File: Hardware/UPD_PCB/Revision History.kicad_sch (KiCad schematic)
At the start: 0 parts

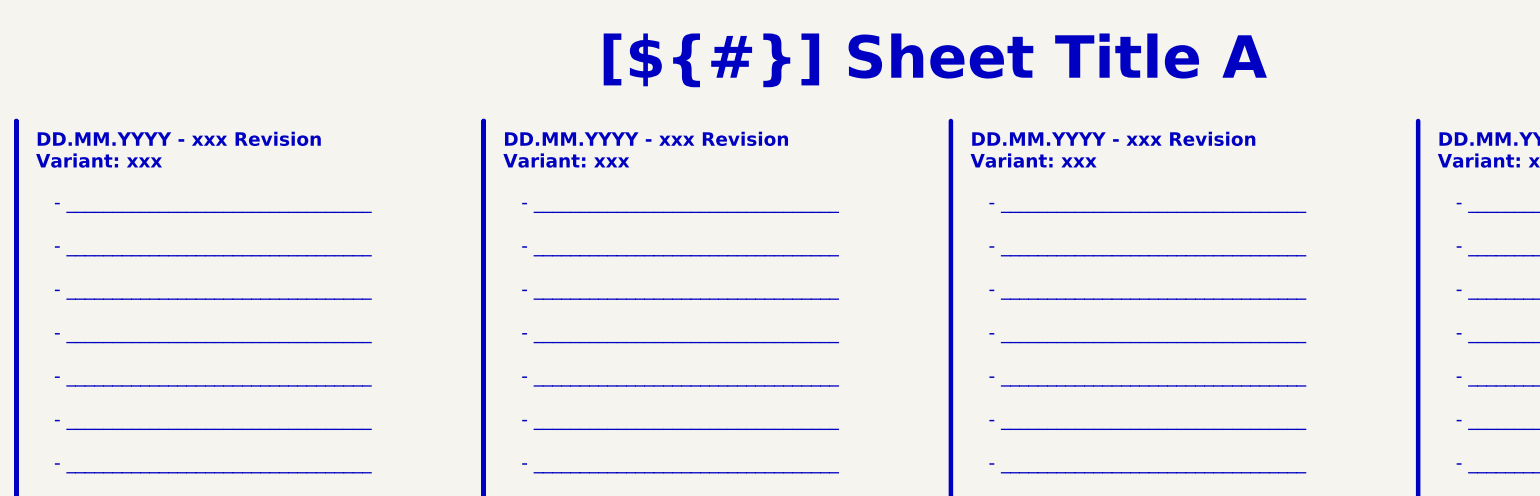
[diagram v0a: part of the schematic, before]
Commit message: Finalized version V1.0
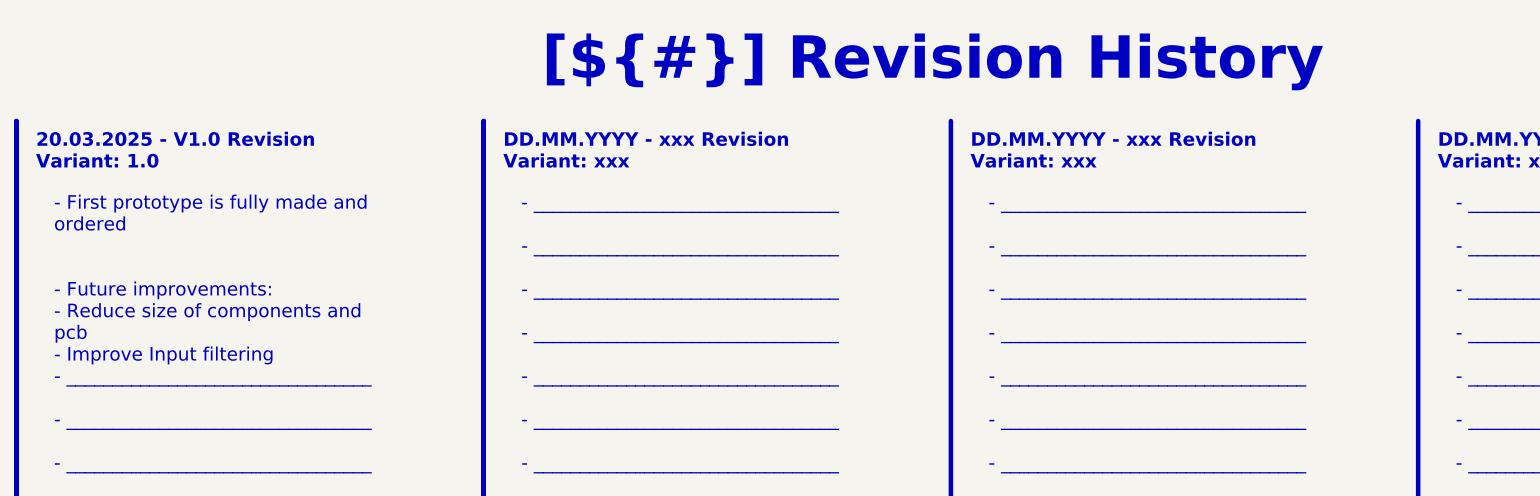
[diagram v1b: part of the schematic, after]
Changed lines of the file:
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@@
 		)
 	)
-	(text_box "[${#}] ${TITLE}"
+	(text_box "[${#}] Revision History\n"
 		(exclude_from_sim no)
 		(at 80.01 16.51 0)
@@
 		)
 	)
-	(text_box "- _________________________________\n\n- _________________________________\n\n- _________________________________\n\n- _________________________________\n\n- _________________________________\n\n- _________________________________\n\n- _________________________________\n\n- _________________________________\n\n- _________________________________\n\n- _________________________________\n\n- _________________________________\n\n- _________________________________\n\n- _________________________________\n\n- _________________________________\n\n- _________________________________\n\n- _________________________________\n\n- _________________________________"
+	(text_box "- First prototype is fully made and ordered\n\n\n- Future improvements:\n- Reduce size of components and pcb\n- Improve Input filtering\n- _________________________________\n\n- _________________________________\n\n- _________________________________\n\n- _________________________________\n\n- _________________________________\n\n- _________________________________\n\n- _________________________________\n\n- _________________________________\n\n- _________________________________\n\n- _________________________________\n\n- _________________________________\n\n- _________________________________\n\n- _________________________________"
 		(exclude_from_sim no)
 		(at 22.86 40.64 0)
@@
 		)
 	)
-	(text_box "DD.MM.YYYY - xxx Revision\nVariant: xxx"
+	(text_box "20.03.2025 - V1.0 Revision\nVariant: 1.0"
 		(exclude_from_sim no)
 		(at 20.32 31.75 0)

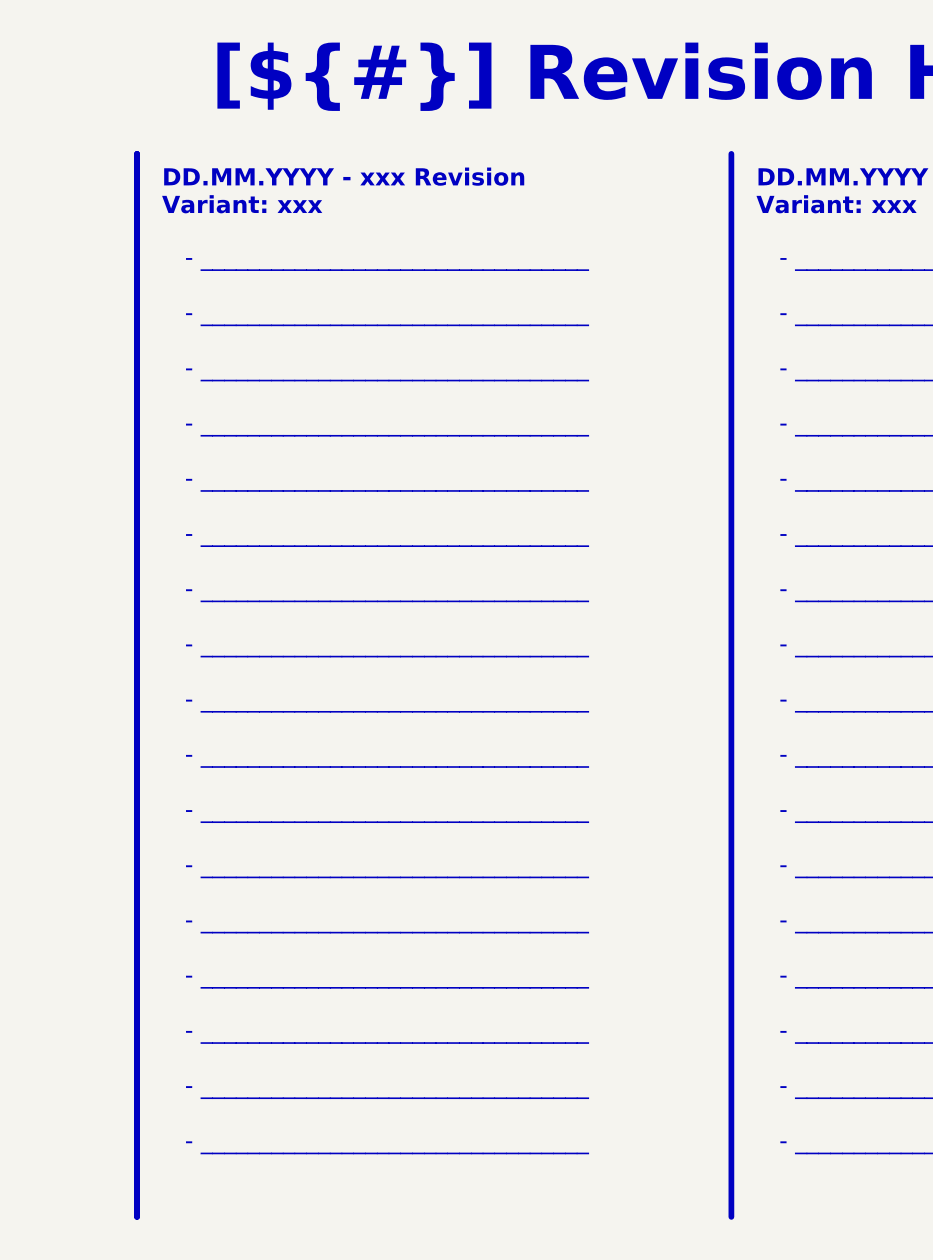
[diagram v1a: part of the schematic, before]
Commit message: Version 1.1 of PCB
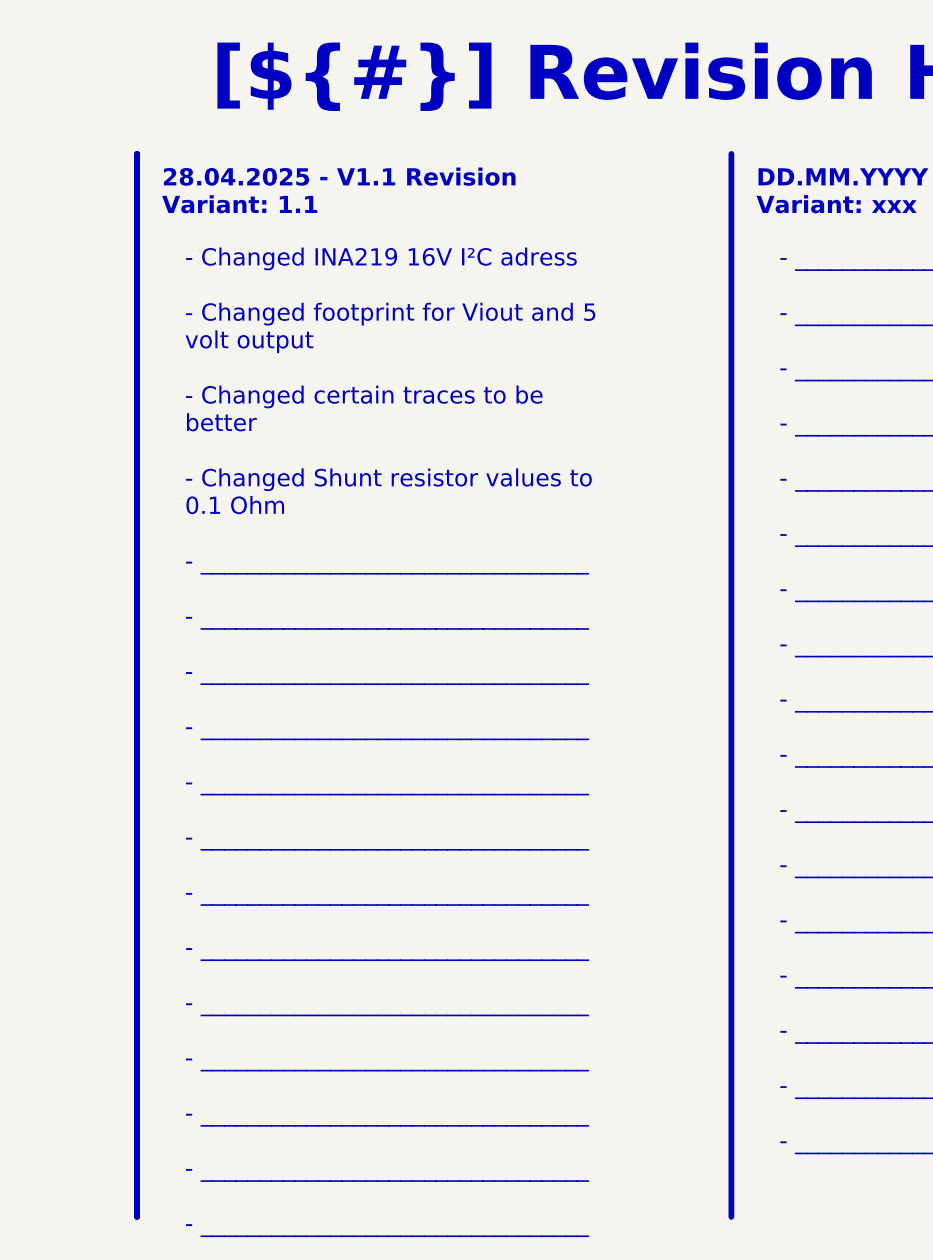
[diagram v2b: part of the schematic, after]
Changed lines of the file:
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@@
 		)
 	)
-	(text_box "DD.MM.YYYY - xxx Revision\nVariant: xxx"
+	(text_box "28.04.2025 - V1.1 Revision\nVariant: 1.1"
 		(exclude_from_sim no)
 		(at 86.36 31.75 0)
@@
 		)
 	)
-	(text_box "- _________________________________\n\n- _________________________________\n\n- _________________________________\n\n- _________________________________\n\n- _________________________________\n\n- _________________________________\n\n- _________________________________\n\n- _________________________________\n\n- _________________________________\n\n- _________________________________\n\n- _________________________________\n\n- _________________________________\n\n- _________________________________\n\n- _________________________________\n\n- _________________________________\n\n- _________________________________\n\n- _________________________________"
+	(text_box "- Changed INA219 16V I²C adress\n\n- Changed footprint for Viout and 5 volt output\n\n- Changed certain traces to be better\n\n- Changed Shunt resistor values to 0.1 Ohm\n\n- _________________________________\n\n- _________________________________\n\n- _________________________________\n\n- _________________________________\n\n- _________________________________\n\n- _________________________________\n\n- _________________________________\n\n- _________________________________\n\n- _________________________________\n\n- _________________________________\n\n- _________________________________\n\n- _________________________________\n\n- _________________________________"
 		(exclude_from_sim no)
 		(at 88.9 40.64 0)
